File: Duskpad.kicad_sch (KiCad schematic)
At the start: 50 parts, among them J1 OLED display, SW1 SW_Push, SW10 SW_Push, SW11 SW_Push, SW12 SW_Push, SW13 SW_Push, SW14 SW_Push, SW15 SW_Push, SW16 SW_Push, SW2 SW_Push, SW3 SW_Push, SW4 SW_Push, SW5 SW_Push, SW6 SW_Push, SW7 SW_Push, SW8 SW_Push, SW9 SW_Push, U1 MOUDLE-SEEEDUINO-XIAO

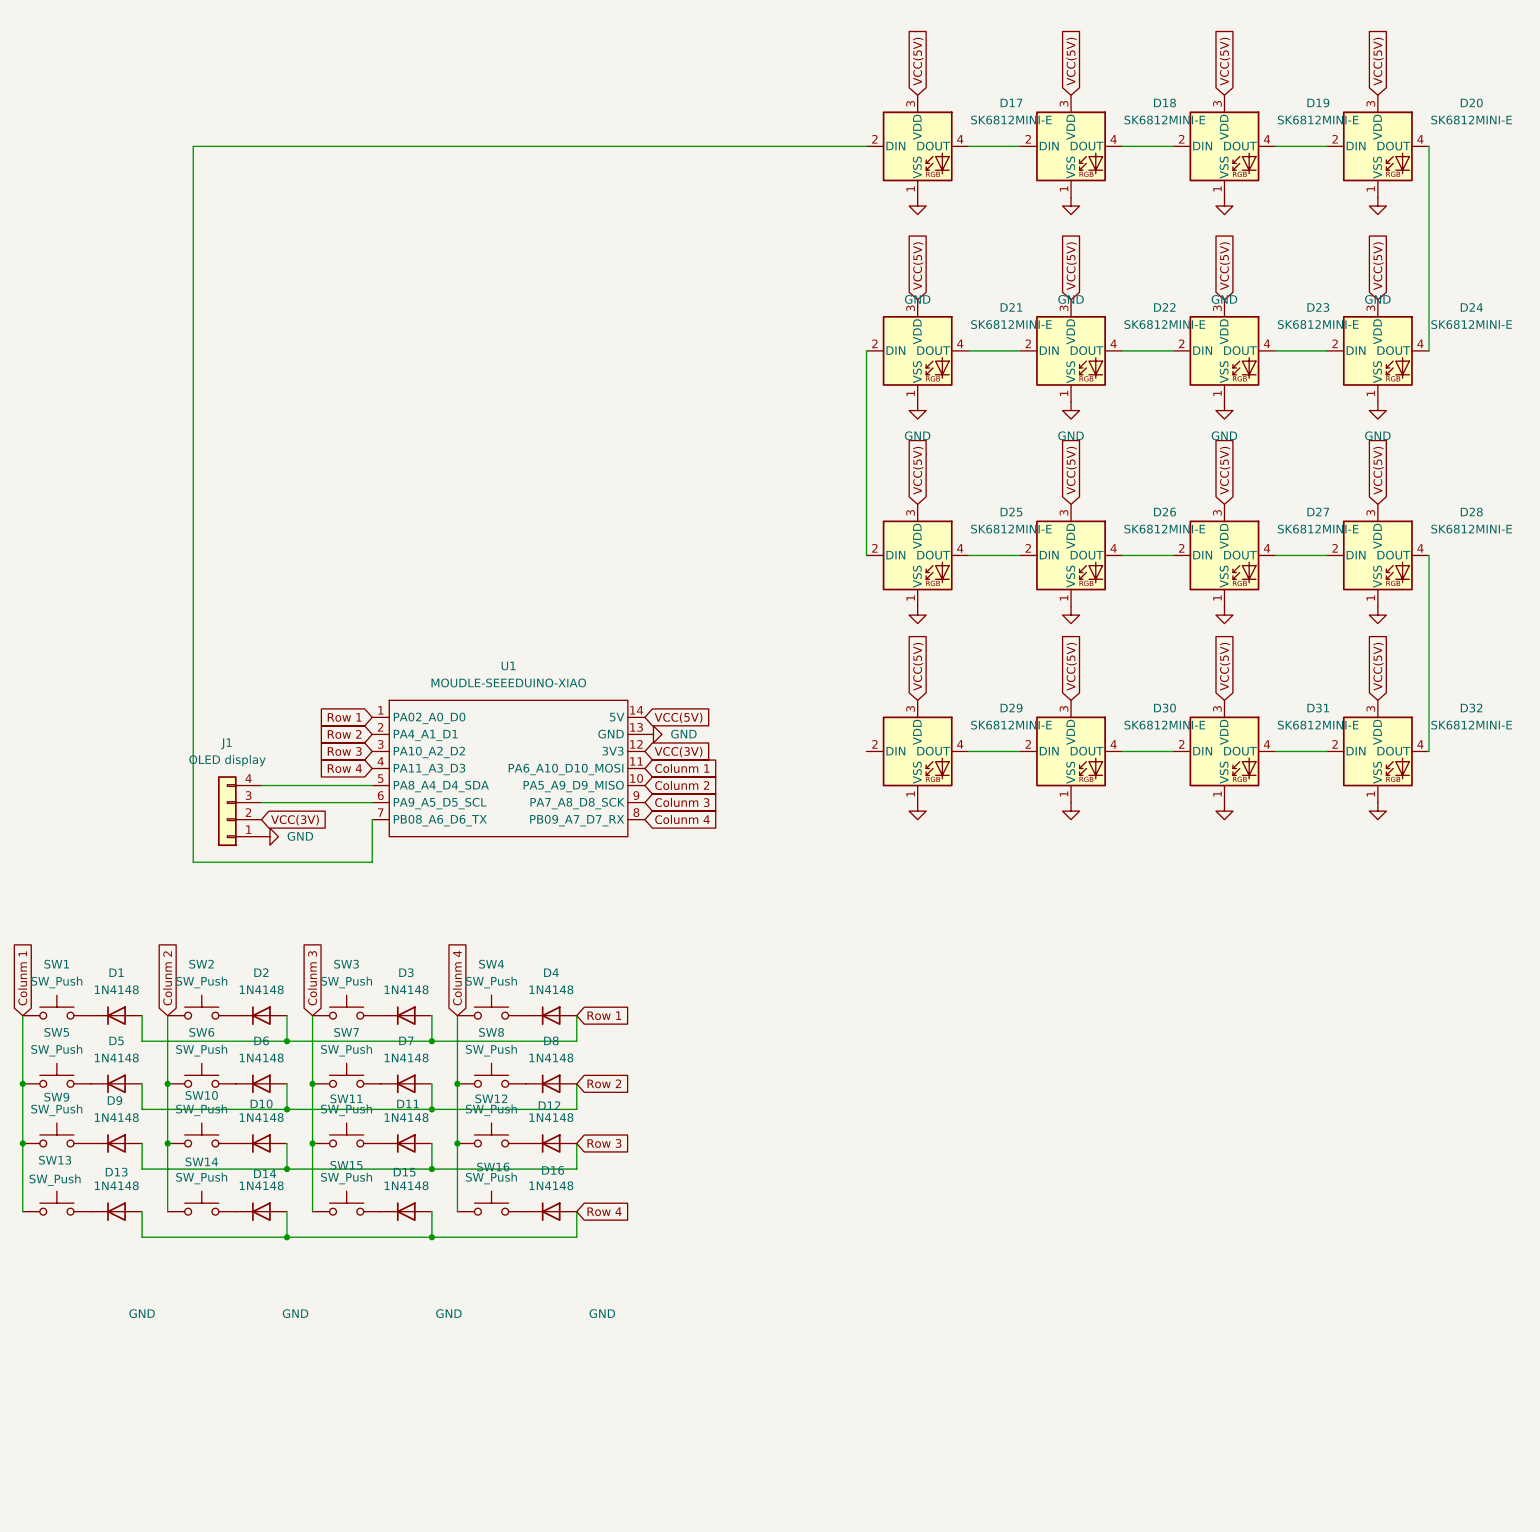
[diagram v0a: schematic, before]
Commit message: did the pcb design
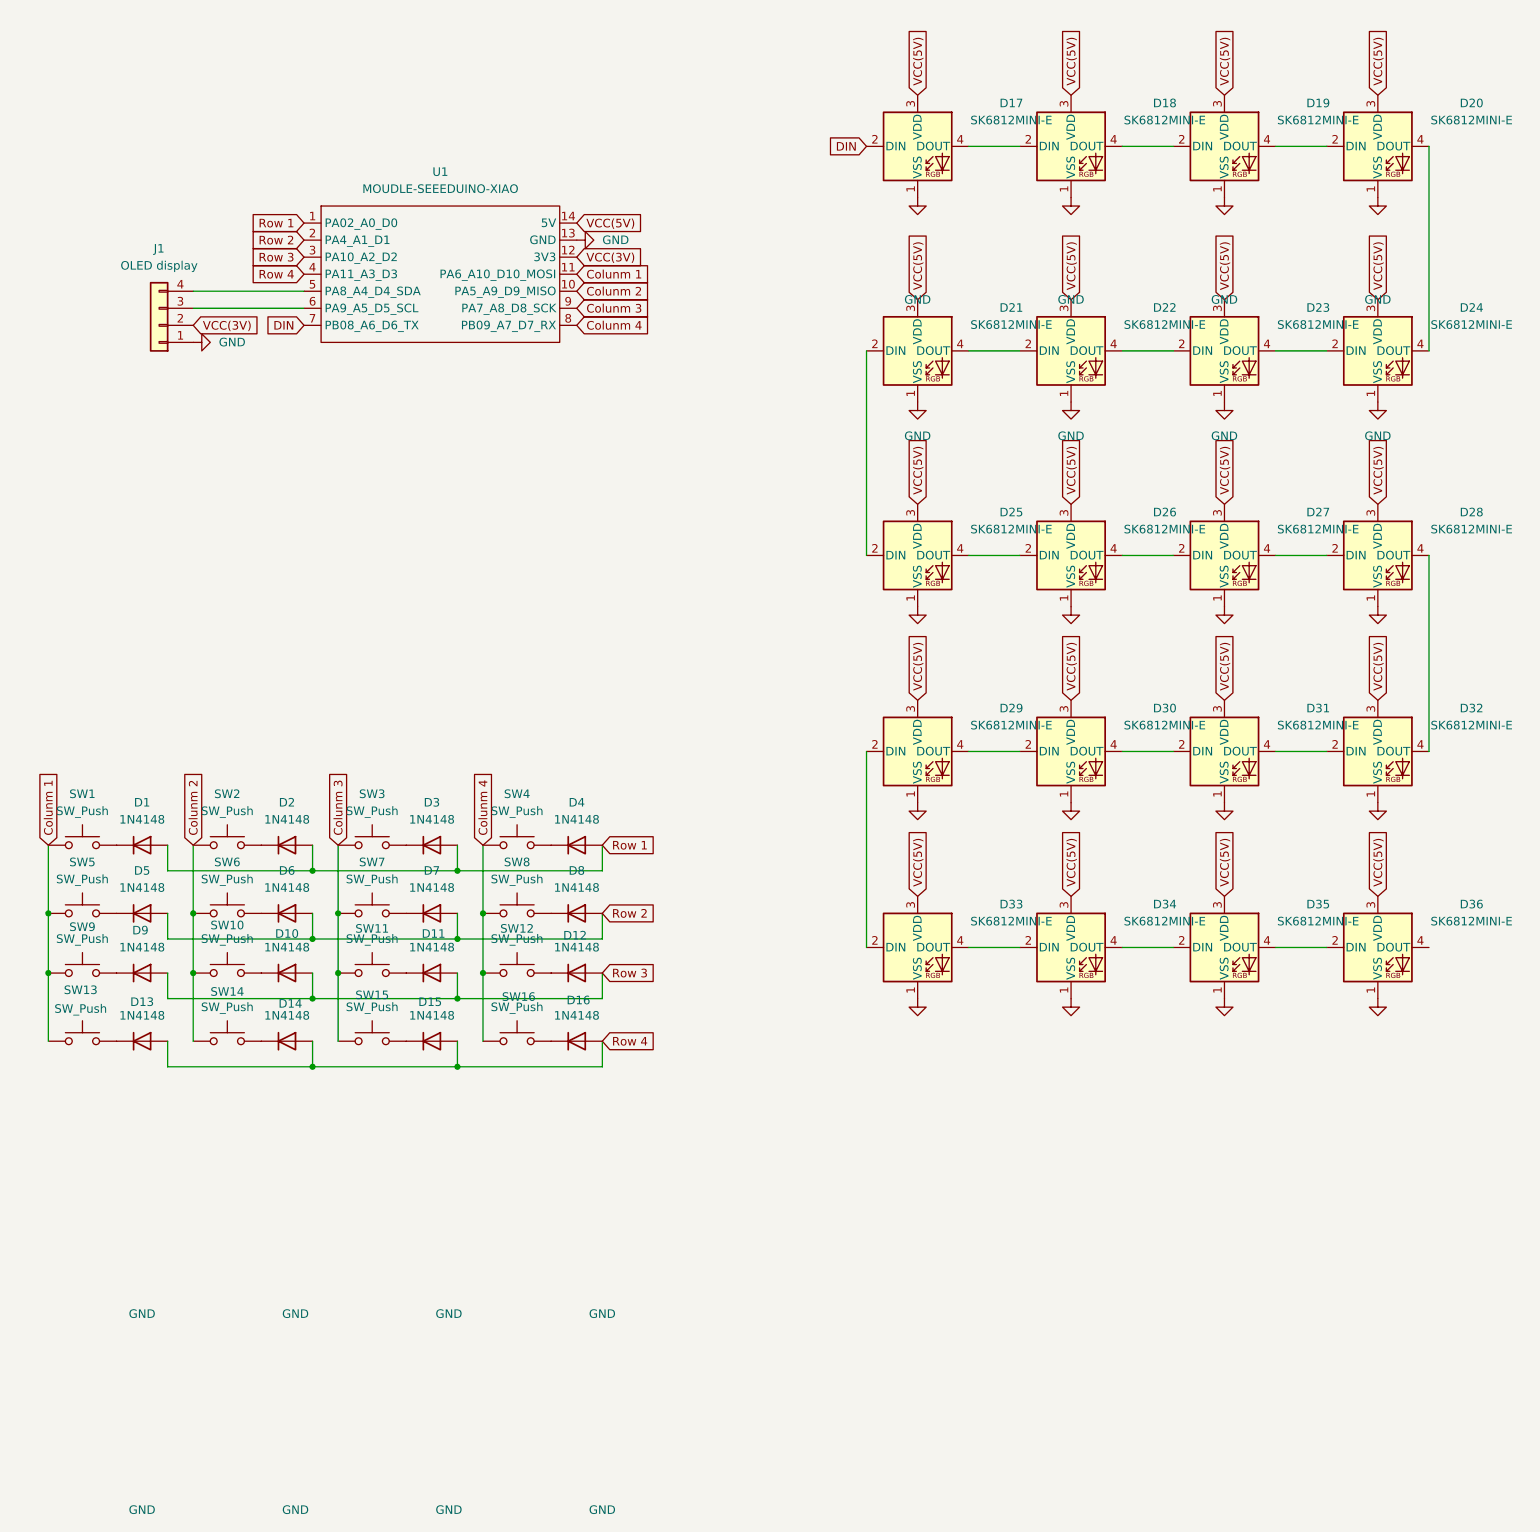
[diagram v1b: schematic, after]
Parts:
- added D33, D34, D35, D36: SK6812MINI-E, LED_SMD:LED_SK6812MINI-E_3.2x2.8mm_P1.5mm_ReverseMount, symbol LED:SK6812MINI-E
- J1: footprint Connector_PinHeader_2.54mm:PinHeader_1x04_P2.54mm_Vertical -> footprints:SSD1306-0.91-OLED-4pin-128x32
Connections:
- net GND: now also D33.1 (VSS), D34.1 (VSS), D35.1 (VSS), D36.1 (VSS)
- net VCC(5V): now also D33.3 (VDD), D34.3 (VDD), D35.3 (VDD), D36.3 (VDD)
- net at D29.2 (DIN): now also D33.2 (DIN)
- net DIN: now reaches D17.2 (DIN), U1.7 (PB08_A6_D6_TX)
- new net: D33.4 (DOUT), D34.2 (DIN)
- new net: D34.4 (DOUT), D35.2 (DIN)
- new net: D35.4 (DOUT), D36.2 (DIN)
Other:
- moved on the sheet: D1, D10, D11, D12, D13, D14, D15, D16, D2, D3, D4, D5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
